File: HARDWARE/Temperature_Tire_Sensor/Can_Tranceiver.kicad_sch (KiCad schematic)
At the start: 2 parts

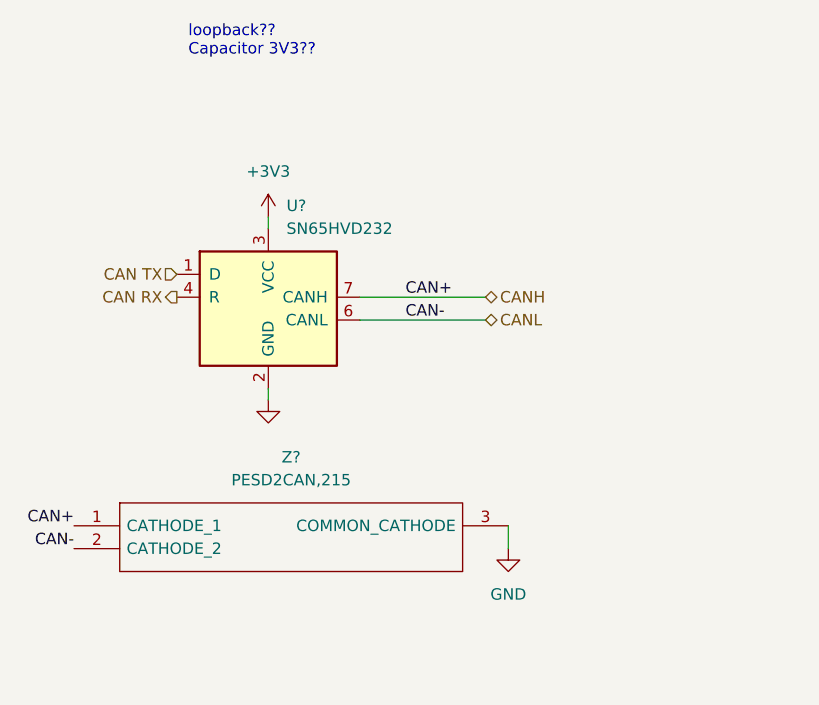
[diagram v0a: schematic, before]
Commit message: A completed schematic
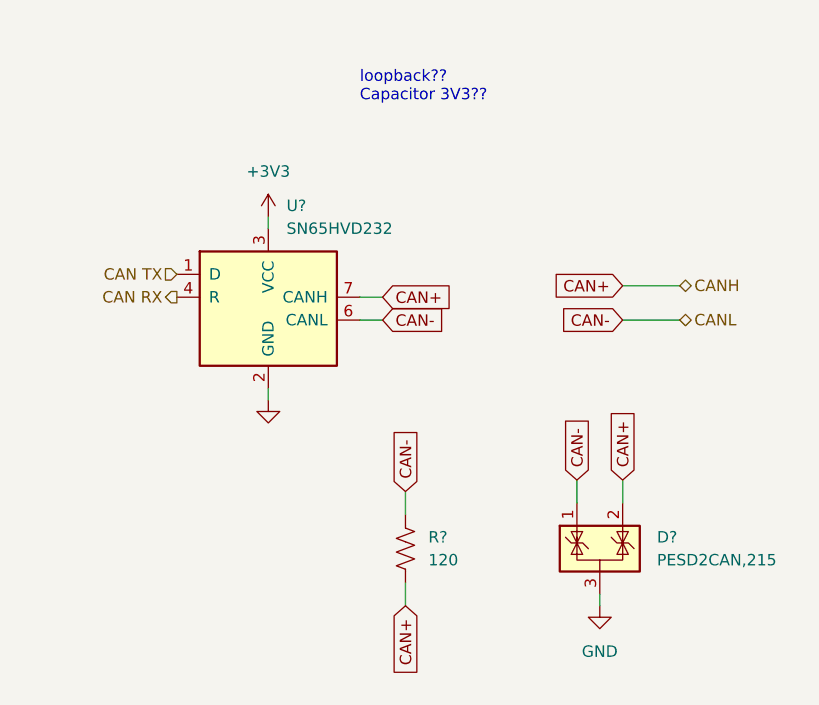
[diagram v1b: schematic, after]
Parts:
- removed Z?: PESD2CAN,215, SOT95P230X110-3N, symbol PESD2CAN_215:PESD2CAN,215
- added D?: PESD2CAN,215, symbol Power_Protection:NUP2105L
- added R?: 120, symbol Device:R_US
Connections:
- net GND: now also D?.3 (A)
- net CANH renamed CAN+
- net CAN+: now also D?.2 (K), R?.2
- net CANL renamed CAN-
- net CAN-: now also D?.1 (K), R?.1
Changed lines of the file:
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@@
     (stroke (width 0) (type default) (color 0 0 0 0))
   )
-  (wire (pts (xy 123.19 91.44) (xy 137.16 91.44))
+  (wire (pts (xy 123.19 91.44) (xy 125.73 91.44))
     (stroke (width 0) (type default) (color 0 0 0 0))
   )
-  (wire (pts (xy 123.19 88.9) (xy 137.16 88.9))
+  (wire (pts (xy 147.32 109.22) (xy 147.32 111.76))
+    (stroke (width 0) (type default) (color 0 0 0 0))
+  )
+  (wire (pts (xy 149.86 121.92) (xy 149.86 123.19))
+    (stroke (width 0) (type default) (color 0 0 0 0))
+  )
+  (wire (pts (xy 123.19 88.9) (xy 125.73 88.9))
+    (stroke (width 0) (type default) (color 0 0 0 0))
+  )
+  (wire (pts (xy 152.4 91.44) (xy 158.75 91.44))
+    (stroke (width 0) (type default) (color 0 0 0 0))
+  )
+  (wire (pts (xy 152.4 87.63) (xy 158.75 87.63))
+    (stroke (width 0) (type default) (color 0 0 0 0))
+  )
+  (wire (pts (xy 152.4 109.22) (xy 152.4 111.76))
     (stroke (width 0) (type default) (color 0 0 0 0))
   )
@@
     (stroke (width 0) (type default) (color 0 0 0 0))
   )
-  (wire (pts (xy 139.7 114.3) (xy 139.7 116.84))
+  (wire (pts (xy 128.27 120.65) (xy 128.27 123.19))
     (stroke (width 0) (type default) (color 0 0 0 0))
   )
-  (text "loopback??\nCapacitor 3V3??" (at 104.14 62.23 0)
+  (wire (pts (xy 128.27 110.49) (xy 128.27 113.03))
+    (stroke (width 0) (type default) (color 0 0 0 0))
+  )
+  (text "loopback??\nCapacitor 3V3??" (at 123.19 67.31 0)
     (effects (font (size 1.27 1.27)) (justify left bottom))
   )
-  (label "CAN+" (at 91.44 114.3 180)
-    (effects (font (size 1.27 1.27)) (justify right bottom))
+  (global_label "CAN+" (shape input) (at 125.73 88.9 0) (fields_autoplaced)
+    (effects (font (size 1.27 1.27)) (justify left))
+    (property "Intersheet References" "${INTERSHEET_REFS}" (id 0) (at 133.4045 88.8206 0)
+      (effects (font (size 1.27 1.27)) (justify left) hide)
+    )
   )
-  (label "CAN-" (at 91.44 116.84 180)
-    (effects (font (size 1.27 1.27)) (justify right bottom))
+  (global_label "CAN+" (shape input) (at 128.27 123.19 270) (fields_autoplaced)
+    (effects (font (size 1.27 1.27)) (justify right))
+    (property "Intersheet References" "${INTERSHEET_REFS}" (id 0) (at 128.1906 130.8645 90)
+      (effects (font (size 1.27 1.27)) (justify right) hide)
+    )
   )
-  (label "CAN+" (at 128.27 88.9 0)
-    (effects (font (size 1.27 1.27)) (justify left bottom))
+  (global_label "CAN-" (shape input) (at 152.4 91.44 180) (fields_autoplaced)
+    (effects (font (size 1.27 1.27)) (justify right))
+    (property "Intersheet References" "${INTERSHEET_REFS}" (id 0) (at 144.7255 91.3606 0)
+      (effects (font (size 1.27 1.27)) (justify right) hide)
+    )
   )
-  (label "CAN-" (at 128.27 91.44 0)
-    (effects (font (size 1.27 1.27)) (justify left bottom))
+  (global_label "CAN+" (shape input) (at 152.4 109.22 90) (fields_autoplaced)
+    (effects (font (size 1.27 1.27)) (justify left))
+    (property "Intersheet References" "${INTERSHEET_REFS}" (id 0) (at 152.4794 101.5455 90)
+      (effects (font (size 1.27 1.27)) (justify left) hide)
+    )
   )
-  (hierarchical_label "CANL" (shape bidirectional) (at 137.16 91.44 0)
+  (global_label "CAN+" (shape input) (at 152.4 87.63 180) (fields_autoplaced)
+    (effects (font (size 1.27 1.27)) (justify right))
+    (property "Intersheet References" "${INTERSHEET_REFS}" (id 0) (at 144.7255 87.5506 0)
+      (effects (font (size 1.27 1.27)) (justify right) hide)
+    )
+  )
+  (global_label "CAN-" (shape input) (at 147.32 109.22 90) (fields_autoplaced)
+    (effects (font (size 1.27 1.27)) (justify left))
+    (property "Intersheet References" "${INTERSHEET_REFS}" (id 0) (at 147.3994 101.5455 90)
+      (effects (font (size 1.27 1.27)) (justify left) hide)
+    )
+  )
+  (global_label "CAN-" (shape input) (at 128.27 110.49 90) (fields_autoplaced)
+    (effects (font (size 1.27 1.27)) (justify left))
+    (property "Intersheet References" "${INTERSHEET_REFS}" (id 0) (at 128.1906 102.8155 90)
+      (effects (font (size 1.27 1.27)) (justify left) hide)
+    )
+  )
+  (global_label "CAN-" (shape input) (at 125.73 91.44 0) (fields_autoplaced)
+    (effects (font (size 1.27 1.27)) (justify left))
+    (property "Intersheet References" "${INTERSHEET_REFS}" (id 0) (at 133.4045 91.3606 0)
+      (effects (font (size 1.27 1.27)) (justify left) hide)
+    )
+  )
+  (hierarchical_label "CANH" (shape bidirectional) (at 158.75 87.63 0)
+    (effects (font (size 1.27 1.27)) (justify left))
+  )
+  (hierarchical_label "CANL" (shape bidirectional) (at 158.75 91.44 0)
     (effects (font (size 1.27 1.27)) (justify left))
   )
@@
     (effects (font (size 1.27 1.27)) (justify right))
   )
-  (hierarchical_label "CANH" (shape bidirectional) (at 137.16 88.9 0)
-    (effects (font (size 1.27 1.27)) (justify left))
-  )
-  (symbol (lib_id "PESD2CAN_215:PESD2CAN,215") (at 91.44 114.3 0) (unit 1)
+  (symbol (lib_id "Power_Protection:NUP2105L") (at 149.86 116.84 0) (unit 1)
     (in_bom yes) (on_board yes) (fields_autoplaced)
-    (property "Reference" "Z?" (id 0) (at 115.57 106.68 0))
-    (property "Value" "PESD2CAN,215" (id 1) (at 115.57 109.22 0))
-    (property "Footprint" "SOT95P230X110-3N" (id 2) (at 135.89 111.76 0)
+    (property "Reference" "D?" (id 0) (at 156.21 115.5699 0)
+      (effects (font (size 1.27 1.27)) (justify left))
+    )
+    (property "Value" "PESD2CAN,215" (id 1) (at 156.21 118.1099 0)
+      (effects (font (size 1.27 1.27)) (justify left))
+    )
+    (property "Footprint" "" (id 2) (at 155.575 118.11 0)
       (effects (font (size 1.27 1.27)) (justify left) hide)
     )
-    (property "Datasheet" "https://datasheet.datasheetarchive.com/originals/distributors/Datasheets_SAMA/5df5edafdc67e6ae251d12d61f18e7bd.pdf" (id 3) (at 135.89 114.3 0)
-      (effects (font (size 1.27 1.27)) (justify left) hide)
+    (property "Datasheet" "" (id 3) (at 153.035 113.665 0)
+      (effects (font (size 1.27 1.27)) hide)
     )
-    (property "Description" "NXP PESD2CAN,215 Dual Bi-Directional ESD Protection Diode, 230W peak, 3-Pin SOT23 (TO-236AB)" (id 4) (at 135.89 116.84 0)
-      (effects (font (size 1.27 1.27)) (justify left) hide)
-    )
-    (property "Height" "1.1" (id 5) (at 135.89 119.38 0)
-      (effects (font (size 1.27 1.27)) (justify left) hide)
-    )
-    (property "Manufacturer_Name" "Nexperia" (id 6) (at 135.89 121.92 0)
-      (effects (font (size 1.27 1.27)) (justify left) hide)
-    )
-    (property "Manufacturer_Part_Number" "PESD2CAN,215" (id 7) (at 135.89 124.46 0)
-      (effects (font (size 1.27 1.27)) (justify left) hide)
-    )
-    (property "Mouser Part Number" "771-PESD2CAN-T/R" (id 8) (at 135.89 127 0)
-      (effects (font (size 1.27 1.27)) (justify left) hide)
-    )
-    (property "Mouser Price/Stock" "https://www.mouser.co.uk/ProductDetail/Nexperia/PESD2CAN215?qs=LOCUfHb8d9sqg7TaLUP2JQ%3D%3D" (id 9) (at 135.89 129.54 0)
-      (effects (font (size 1.27 1.27)) (justify left) hide)
-    )
-    (property "Arrow Part Number" "PESD2CAN,215" (id 10) (at 135.89 132.08 0)
-      (effects (font (size 1.27 1.27)) (justify left) hide)
-    )
-    (property "Arrow Price/Stock" "https://www.arrow.com/en/products/pesd2can215/nexperia?region=nac" (id 11) (at 135.89 134.62 0)
-      (effects (font (size 1.27 1.27)) (justify left) hide)
-    )
+    (pin "3")
     (pin "1")
     (pin "2")
-    (pin "3")
   )
   (symbol (lib_id "power:GND") (at 113.03 100.33 0) (unit 1)
-    (in_bom yes) (on_board yes) (fields_autoplaced)
+    (in_bom yes) (on_board yes)
     (property "Reference" "#PWR?" (id 0) (at 113.03 106.68 0)
       (effects (font (size 1.27 1.27)) hide)
     )
-    (property "Value" "~" (id 1) (at 113.03 105.41 0))
+    (property "Value" "~" (id 1) (at 119.38 111.76 0))
     (property "Footprint" "" (id 2) (at 113.03 100.33 0)
       (effects (font (size 1.27 1.27)) hide)
@@
     (pin "1")
   )
-  (symbol (lib_id "power:GND") (at 139.7 116.84 0) (unit 1)
+  (symbol (lib_id "power:GND") (at 149.86 123.19 0) (unit 1)
     (in_bom yes) (on_board yes) (fields_autoplaced)
-    (property "Reference" "#PWR?" (id 0) (at 139.7 123.19 0)
+    (property "Reference" "#PWR?" (id 0) (at 149.86 129.54 0)
       (effects (font (size 1.27 1.27)) hide)
     )
-    (property "Value" "GND" (id 1) (at 139.7 121.92 0))
-    (property "Footprint" "" (id 2) (at 139.7 116.84 0)
+    (property "Value" "GND" (id 1) (at 149.86 128.27 0))
+    (property "Footprint" "" (id 2) (at 149.86 123.19 0)
       (effects (font (size 1.27 1.27)) hide)
     )
-    (property "Datasheet" "" (id 3) (at 139.7 116.84 0)
+    (property "Datasheet" "" (id 3) (at 149.86 123.19 0)
       (effects (font (size 1.27 1.27)) hide)
     )
@@
     (pin "1")
   )
+  (symbol (lib_id "Device:R_US") (at 128.27 116.84 0) (unit 1)
+    (in_bom yes) (on_board yes) (fields_autoplaced)
+    (property "Reference" "R?" (id 0) (at 130.81 115.5699 0)
+      (effects (font (size 1.27 1.27)) (justify left))
+    )
+    (property "Value" "120" (id 1) (at 130.81 118.1099 0)
+      (effects (font (size 1.27 1.27)) (justify left))
+    )
+    (property "Footprint" "" (id 2) (at 129.286 117.094 90)
+      (effects (font (size 1.27 1.27)) hide)
+    )
+    (property "Datasheet" "~" (id 3) (at 128.27 116.84 0)
+      (effects (font (size 1.27 1.27)) hide)
+    )
+    (pin "1")
+    (pin "2")
+  )
   (symbol (lib_id "Interface_CAN_LIN:SN65HVD232") (at 113.03 88.9 0) (unit 1)
